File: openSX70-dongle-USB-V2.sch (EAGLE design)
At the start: 25 parts, among them J1 687106183722, J2 SJ-3523-SMT-TR, U1 FT232RLSSOP

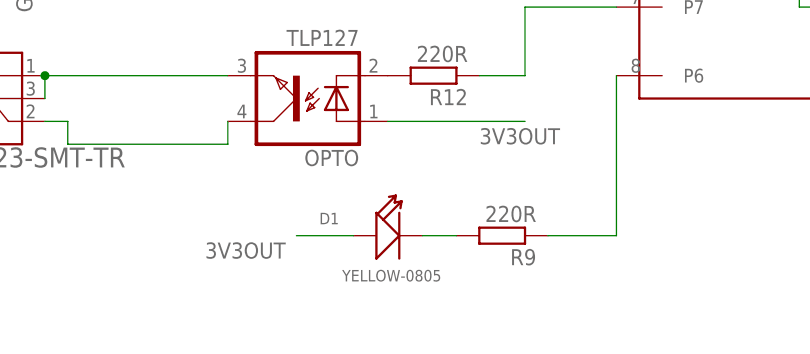
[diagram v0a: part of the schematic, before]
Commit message: new origami design
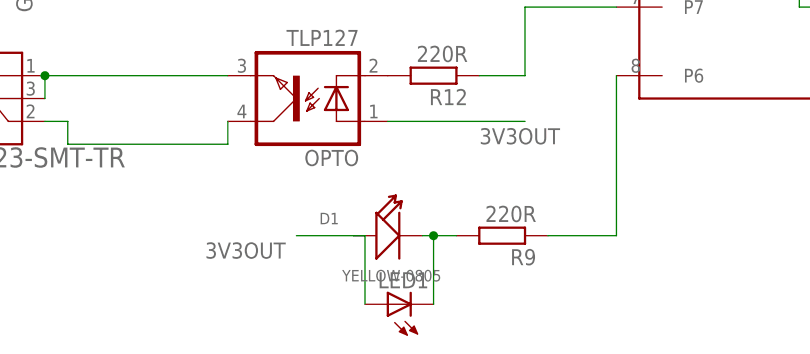
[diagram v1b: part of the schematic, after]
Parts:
- added LED1: (no value), openSX70_PATHFINDER_V5.5-SEEED_20180522:LED3MM
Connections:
- net 3V3OUT: now also LED1.A
- net N$2: now also LED1.C
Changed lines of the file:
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@@
 <part name="D1" library="Seeed-LED-2016" deviceset="SMD-LED-CLEAR-YELLOW(0805)" device="" value="YELLOW-0805"/>
 <part name="U$5" library="_openSX70" deviceset="DUOLED-PROPER-LTST-C195KGJRKT" device=""/>
+<part name="LED1" library="openSX70_PATHFINDER_V5.5-SEEED_20180522" deviceset="LED" device="3MM"/>
 </parts>
 <sheets>
@@
 <attribute name="NAME" x="185.42" y="137.92631875" size="1.779309375" layer="95" rot="MR0"/>
 <attribute name="VALUE" x="185.42" y="140.0882" size="1.7796" layer="96" rot="MR0"/>
+</instance>
+<instance part="LED1" gate="G$1" x="45.72" y="-10.16" rot="R90">
+<attribute name="NAME" x="50.292" y="-6.604" size="1.778" layer="95" rot="R180"/>
+<attribute name="VALUE" x="50.292" y="-4.445" size="1.778" layer="96" rot="R180"/>
 </instance>
 </instances>
@@
 <segment>
 <pinref part="D1" gate="G$1" pin="+"/>
+<label x="25.4" y="-5.08" size="1.778" layer="95"/>
+<pinref part="LED1" gate="G$1" pin="A"/>
 <wire x1="41.91" y1="-2.54" x2="35.56" y2="-2.54" width="0.1524" layer="91"/>
-<label x="25.4" y="-5.08" size="1.778" layer="95"/>
+<wire x1="41.91" y1="-2.54" x2="43.18" y2="-2.54" width="0.1524" layer="91"/>
+<wire x1="43.18" y1="-2.54" x2="43.18" y2="-10.16" width="0.1524" layer="91"/>
 </segment>
 </net>
@@
 <pinref part="D1" gate="G$1" pin="-"/>
 <pinref part="R9" gate="G$1" pin="2"/>
-<wire x1="49.53" y1="-2.54" x2="53.34" y2="-2.54" width="0.1524" layer="91"/>
-</segment>
-</net>
+<wire x1="49.53" y1="-2.54" x2="50.8" y2="-2.54" width="0.1524" layer="91"/>
+<pinref part="LED1" gate="G$1" pin="C"/>
+<wire x1="50.8" y1="-2.54" x2="53.34" y2="-2.54" width="0.1524" layer="91"/>
+<wire x1="50.8" y1="-10.16" x2="50.8" y2="-2.54" width="0.1524" layer="91"/>
+<junction x="50.8" y="-2.54"/>
+</segment>
+</net>
